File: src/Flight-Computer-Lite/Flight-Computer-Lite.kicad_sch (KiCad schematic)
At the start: 39 parts, among them J1 Jumper_NO, J2 Jumper_NO, P1 1546551-2, P2 3220-20-0200-00, U1 STM32H750VBTx, U2 LMS8117AMP-3.3_NOPB, Y1 ECS-240-18-33-JGN-TR

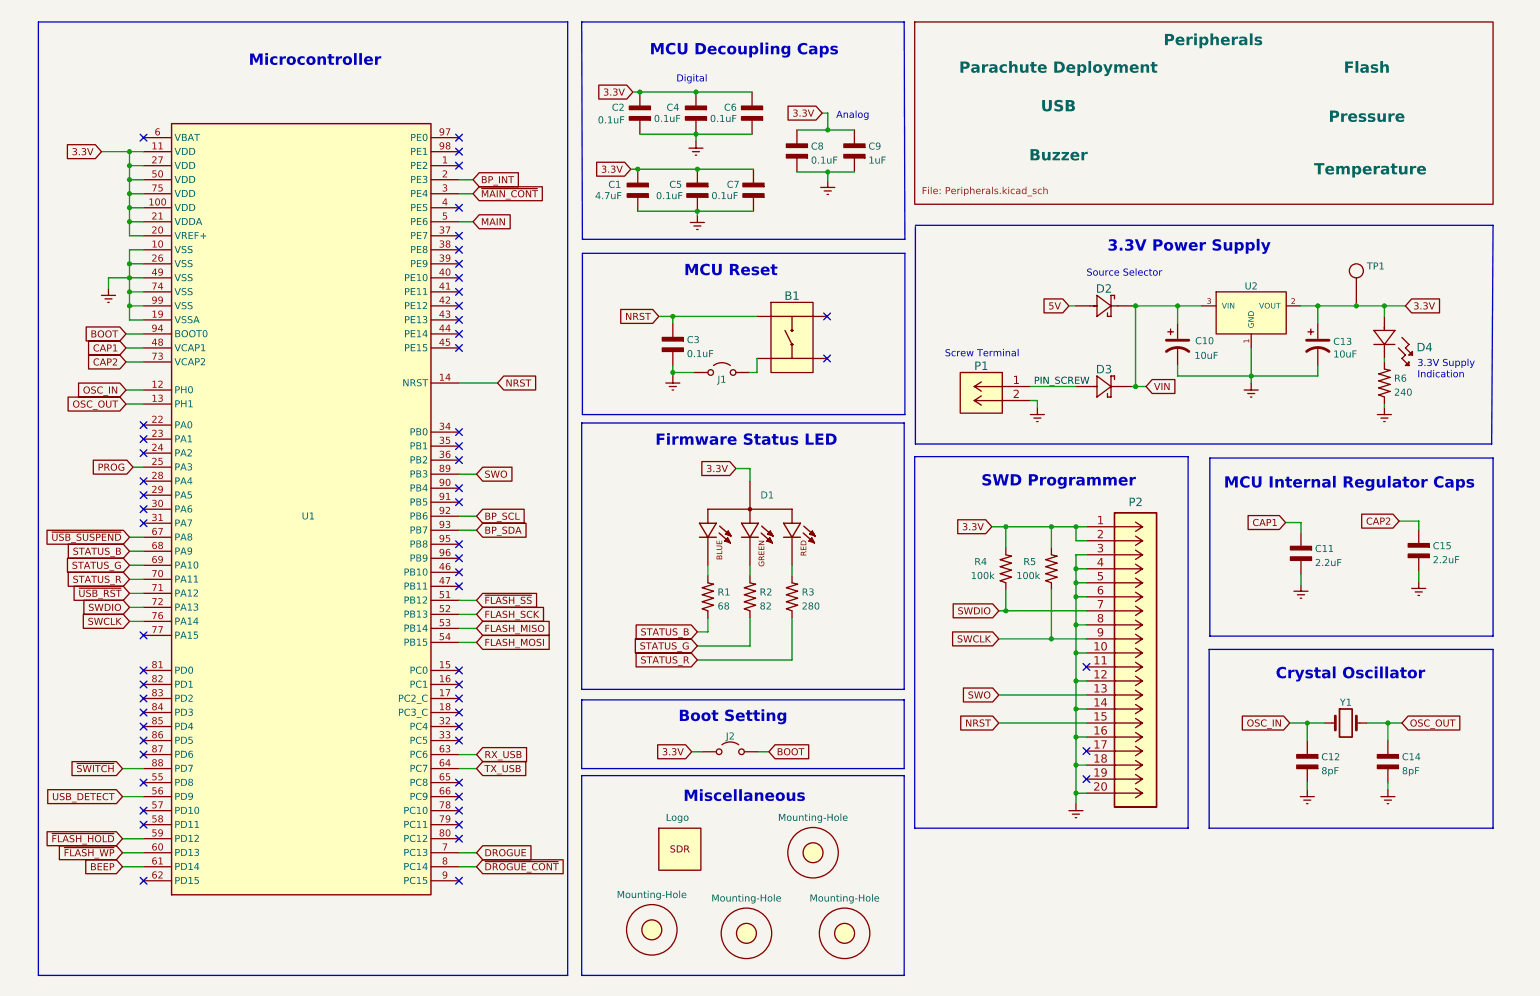
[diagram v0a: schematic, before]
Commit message: created rev2 schematic
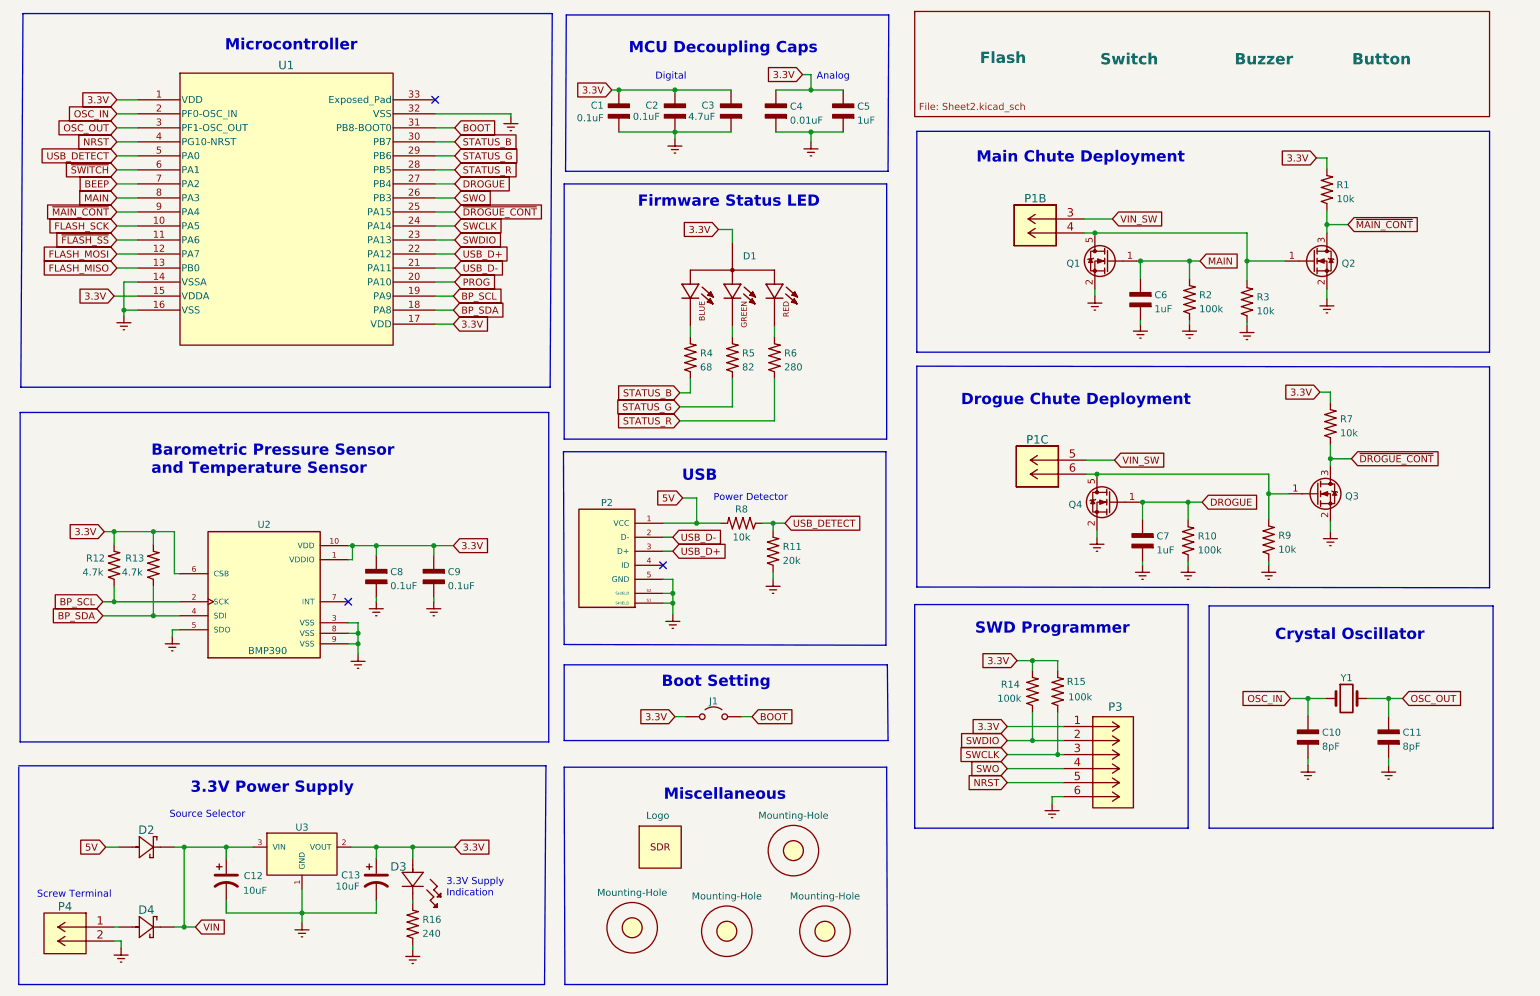
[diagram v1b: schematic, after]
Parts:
- removed B1: PTS647SM38SMTR2LFS, Flight-Computer:PTS647SM38SMTR2LFS, symbol Flight-Computer:PTS647SM38SMTR2LFS
- removed C11, C15: 2.2uF, Flight-Computer-Lite:CAP_0603, symbol Flight-Computer:CAP_0603
- removed C3, C5: 0.1uF, Flight-Computer-Lite:CAP_0603, symbol Flight-Computer:CAP_0603
- removed J1: Jumper_NO, Flight-Computer-Lite:Jumper-NO, symbol Flight-Computer:Jumper_NO
- removed P2: 3220-20-0200-00, Flight-Computer-Lite:3220-20-0200-00, symbol Flight-Computer:3220-20-0200-00
- removed TP1: TP, Flight-Computer-Lite:TP, symbol Flight-Computer:TP
- removed U1: STM32H750VBTx, Flight-Computer-Lite:STM32H750VBT6, symbol Flight-Computer-Lite:STM32H750VBTx
- added C8, C9: 0.1uF, Flight-Computer-Lite:CAP_0603, symbol Flight-Computer:CAP_0603
- added P1: 1984659, Flight-Computer-Lite:1984659, symbol Flight-Computer:1984659
- added P2: USB, Flight-Computer-Lite:10118194-0001LF, symbol Flight-Computer-Lite:USB
- added P3: 0530470610, Flight-Computer-Lite:53047-0610, symbol Flight-Computer-Lite:0530470610
- added Q1, Q4: QS5U17TR, Flight-Computer-Lite:QS5U17TR, symbol Flight-Computer:QS5U17TR
- added Q2, Q3: 2N7002W-7-F, Flight-Computer-Lite:2N7002W-7-F, symbol Flight-Computer-Lite:2N7002W-7-F
- added R1, R3, R7, R8, R9: 10k, Flight-Computer-Lite:RES_0603, symbol Flight-Computer:RES_0603
- added R10, R2: 100k, Flight-Computer-Lite:RES_0603, symbol Flight-Computer:RES_0603
- added R11: 20k, Flight-Computer-Lite:RES_0603, symbol Flight-Computer:RES_0603
- added R12, R13: 4.7k, Flight-Computer-Lite:RES_0603, symbol Flight-Computer:RES_0603
- added U1: STM32G4A1KEU6, Flight-Computer-Lite:STM32G4A1KEU6, symbol Flight-Computer-Lite:STM32G4A1KEU6
- added U2: BMP390, Flight-Computer-Lite:BMP390, symbol Flight-Computer:BMP390
- C4: renamed from C8; value 0.1uF -> 0.01uF
- C6, C7: value 0.1uF -> 1uF
- renumbered C2 to C1, C12 to C10, C14 to C11, C10 to C12, C4 to C2, C1 to C3, C9 to C5, D4 to D3, D3 to D4, H2 to H1, H1 to H2, H4 to H3, H3 to H4, J2 to J1, P1 to P4, R4 to R14, R5 to R15, R6 to R16, R1 to R4, R2 to R5, R3 to R6, U2 to U3
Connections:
- net 3.3V: now also C8.1, C9.1, P3.1, R1.2, R12.2, R13.2, R7.2, U1.1 (VDD), U1.15 (VDDA), U1.17 (VDD), U2.1 (VDDIO), U2.10 (VDD), U2.6 (CSB); no longer C6.1, C7.1
- net 5V: now also P2.1 (VCC), R8.2
- net BEEP: now also U1.7 (PA2)
- net BOOT: now also U1.31 (PB8-BOOT0)
- net BP_SCL: now also R12.1, U1.19 (PA9), U2.2 (SCK)
- net BP_SDA: now also R13.1, U1.18 (PA8), U2.4 (SDI)
- net DROGUE: now also C7.1, Q4.1 (G), R10.2, U1.27 (PB4)
- net Earth: now also C8.2, C9.2, P2.5 (GND), P2.S1 (SHIELD), P2.S2 (SHIELD), P3.6, Q1.2 (S), Q2.2 (S), Q3.2 (S), Q4.2 (S), R10.1, R11.1, R2.1, R3.1, R9.1, U1.14 (VSSA), U1.16 (VSS), U1.32 (VSS), U2.3 (VSS), U2.5 (SDO), U2.8 (VSS), U2.9 (VSS)
- net FLASH_MISO: now also U1.13 (PB0)
- net FLASH_MOSI: now also U1.12 (PA7)
- net FLASH_SCK: now also U1.10 (PA5)
- net MAIN: now also C6.1, Q1.1 (G), R2.2, U1.8 (PA3)
- net NRST: now also P3.5, U1.4 (PG10-NRST)
- net OSC_IN: now also U1.2 (PF0-OSC_IN)
- net OSC_OUT: now also U1.3 (PF1-OSC_OUT)
- net PROG: now also U1.20 (PA10)
- net STATUS_B: now also U1.30 (PB7)
- net STATUS_G: now also U1.29 (PB6)
- net STATUS_R: now also U1.28 (PB5)
- net SWCLK: now also P3.3, U1.24 (PA14)
- net SWDIO: now also P3.2, U1.23 (PA13)
- net SWO: now also P3.4, U1.26 (PB3)
- net USB_DETECT: now also R11.2, R8.1, U1.5 (PA0)
- net ~{DROGUE_CONT}: now also Q3.3 (D), R7.1, U1.25 (PA15)
- net ~{FLASH_SS}: now also U1.11 (PA6)
- net ~{MAIN_CONT}: now also Q2.3 (D), R1.1, U1.9 (PA4)
- net ~{SWITCH}: now also U1.6 (PA1)
- net PIN_SCREW: no longer names the net of D4.2, P4.1 (5)
- new net: P1.4 (6), Q1.5 (D), Q2.1 (G), R3.2
- new net: P1.6, Q3.1 (G), Q4.5 (D), R9.2
- new net USB_D+: P2.3 (D+), U1.22 (PA12)
- new net USB_D-: P2.2 (D-), U1.21 (PA11)
- new net VIN_SW: P1.3 (5), P1.5
- no-connect marks 59 -> 3
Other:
- removed sheet Peripherals
- added sheet Sheet2 (Sheet2.kicad_sch)
- note added: "Barometric Pressure Sensor and Temperature Sensor"
- note added: "Drogue Chute Deployment"
- note added: "Main Chute Deployment"
- note added: "Power Detector"
- note added: "USB"
- note removed: "MCU Internal Regulator Caps"
- note removed: "MCU Reset"
- moved on the sheet: C1, C10, C11, C12, C13, C2, C3, C4, C5, D1, D2, D3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
